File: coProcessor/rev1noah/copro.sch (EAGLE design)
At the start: 97 parts, among them IC1 STM32F405RGT6, J1 USB_MINI-B_SMT, J2 79107-08, J3 693061010911, J4 30320-6002HB, T1 2N2222, T10 2N2222, T2 2N2222, T3 2N2222, T4 2N2222, T5 2N2222, T6 2N2222, T7 2N2222, T8 2N2222, T9 2N2222, U1 LM2597N-5.0, U2 SN65HVD232QD

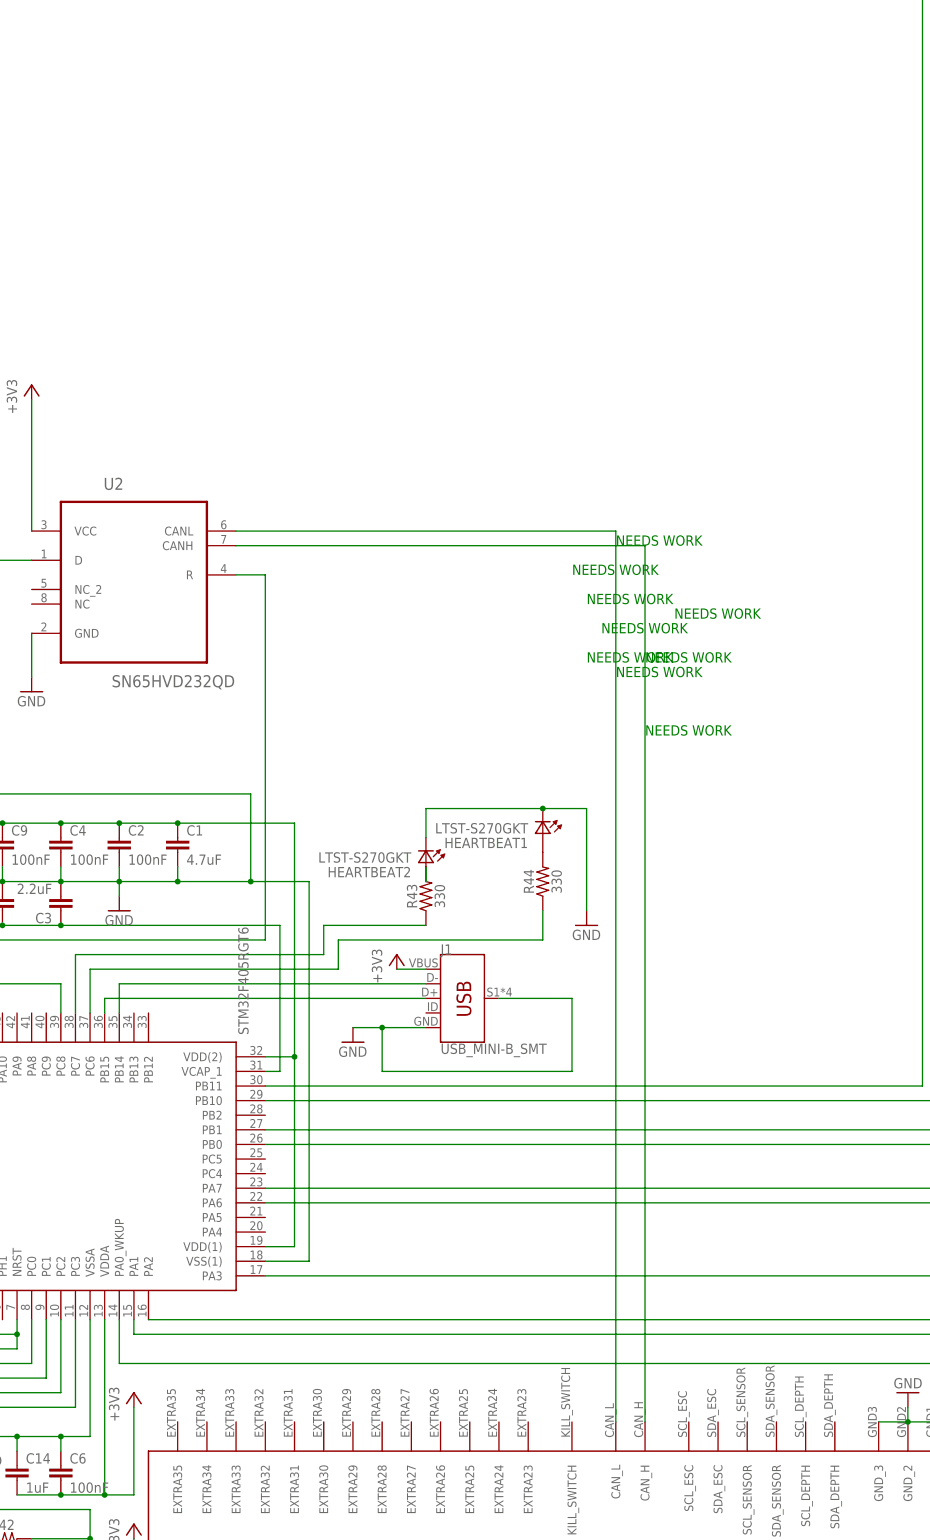
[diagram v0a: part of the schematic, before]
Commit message: Slight progress on last commit, just so everything is up to date
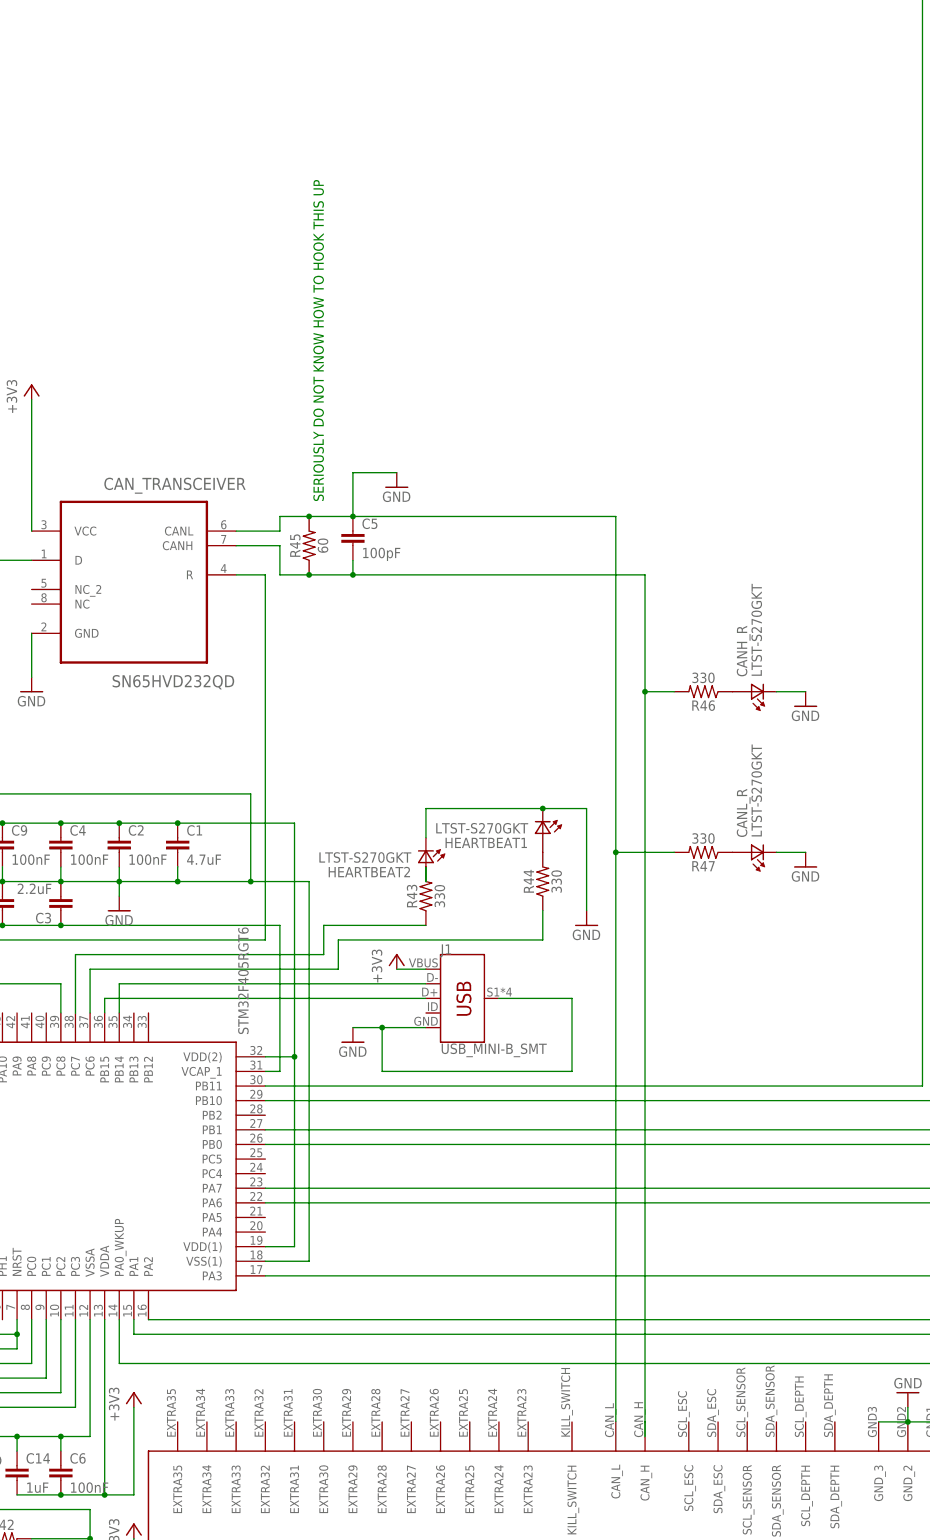
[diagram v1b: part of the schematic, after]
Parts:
- added C5: 100pF, SparkFun-Capacitors:0.1UF-0603-100V-10%
- added CANH_R, CANL_R: LTST-S270GKT, LTST-S270GKT:LTST-S270GKT
- added R45: 60, SparkFun-Resistors:1KOHM-0603-1/10W-1%
- added R46, R47: 330, SparkFun-Resistors:1KOHM-0603-1/10W-1%
- renumbered U2 to CAN_TRANSCEIVER
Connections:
- net N$5 renamed RXD
- removed net N$12: CAN_TRANSCEIVER.CANL, U$1.CAN_L
- new net CANH: C5.2, CAN_TRANSCEIVER.CANH, R45.1, R46.2, U$1.CAN_H
- new net CANL: C5.1, CAN_TRANSCEIVER.CANL, R45.2, R47.2, U$1.CAN_L
- new net N$34: CANH_R.A2, R46.1
- net GND: now also CANH_R.K2, CANL_R.K2
- net N$8: now also CANL_R.A2, R47.1; no longer CAN_TRANSCEIVER.CANH, U$1.CAN_H
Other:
- note added: "SERIOUSLY DO NOT KNOW HOW TO HOOK THIS UP"
- note removed: "NEEDS WORK"
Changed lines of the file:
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@@
 <part name="GND29" library="supply1" library_urn="urn:adsk.eagle:library:371" deviceset="GND" device=""/>
 <part name="+3V3" library="supply1" library_urn="urn:adsk.eagle:library:371" deviceset="+3V3" device=""/>
-<part name="U2" library="SN65HVD232QD" deviceset="SN65HVD232QD" device=""/>
+<part name="CAN_TRANSCEIVER" library="SN65HVD232QD" deviceset="SN65HVD232QD" device=""/>
 <part name="J2" library="con-molex-milli-grid" deviceset="79107-08" device=""/>
 <part name="+3V9" library="supply1" library_urn="urn:adsk.eagle:library:371" deviceset="+3V3" device=""/>
+<part name="R45" library="SparkFun-Resistors" deviceset="1KOHM" device="-0603-1/10W-1%" value="60"/>
+<part name="C5" library="SparkFun-Capacitors" deviceset="0.1UF" device="-0603-100V-10%" value="100pF"/>
+<part name="GND30" library="supply1" library_urn="urn:adsk.eagle:library:371" deviceset="GND" device=""/>
+<part name="R46" library="SparkFun-Resistors" deviceset="1KOHM" device="-0603-1/10W-1%" value="330"/>
+<part name="R47" library="SparkFun-Resistors" deviceset="1KOHM" device="-0603-1/10W-1%" value="330"/>
+<part name="CANL_R" library="LTST-S270GKT" deviceset="LTST-S270GKT" device=""/>
+<part name="CANH_R" library="LTST-S270GKT" deviceset="LTST-S270GKT" device=""/>
+<part name="GND31" library="supply1" library_urn="urn:adsk.eagle:library:371" deviceset="GND" device=""/>
+<part name="GND32" library="supply1" library_urn="urn:adsk.eagle:library:371" deviceset="GND" device=""/>
 </parts>
 <sheets>
@@
 <text x="426.72" y="38.1" size="1.778" layer="91">5 v</text>
 <text x="408.94" y="71.12" size="1.778" layer="91">18 - 22 V</text>
-<text x="279.4" y="226.06" size="1.778" layer="91">NEEDS WORK</text>
-<text x="274.32" y="236.22" size="1.778" layer="91">NEEDS WORK</text>
-<text x="276.86" y="220.98" size="1.778" layer="91">NEEDS WORK</text>
-<text x="287.02" y="208.28" size="1.778" layer="91">NEEDS WORK</text>
-<text x="276.86" y="231.14" size="1.778" layer="91">NEEDS WORK</text>
-<text x="281.94" y="241.3" size="1.778" layer="91">NEEDS WORK</text>
-<text x="292.1" y="228.6" size="1.778" layer="91">NEEDS WORK</text>
-<text x="287.02" y="220.98" size="1.778" layer="91">NEEDS WORK</text>
-<text x="281.94" y="218.44" size="1.778" layer="91">NEEDS WORK</text>
+<text x="231.14" y="248.92" size="1.778" layer="91" rot="R90">SERIOUSLY DO NOT KNOW HOW TO HOOK THIS UP</text>
 </plain>
 <instances>
@@
 <instance part="GND29" gate="1" x="180.34" y="215.9"/>
 <instance part="+3V3" gate="G$1" x="180.34" y="269.24"/>
-<instance part="U2" gate="A" x="198.12" y="238.76"/>
+<instance part="CAN_TRANSCEIVER" gate="A" x="198.12" y="238.76"/>
 <instance part="J2" gate="G$1" x="91.44" y="66.04" rot="R90"/>
 <instance part="+3V9" gate="G$1" x="76.2" y="63.5"/>
+<instance part="R45" gate="G$1" x="228.6" y="241.3" rot="R90"/>
+<instance part="C5" gate="G$1" x="236.22" y="241.3"/>
+<instance part="GND30" gate="1" x="243.84" y="251.46"/>
+<instance part="R46" gate="G$1" x="297.18" y="215.9" rot="R180"/>
+<instance part="R47" gate="G$1" x="297.18" y="187.96" rot="R180"/>
+<instance part="CANL_R" gate="G$1" x="307.34" y="187.96" rot="R90"/>
+<instance part="CANH_R" gate="G$1" x="307.34" y="215.9" rot="R90"/>
+<instance part="GND31" gate="1" x="314.96" y="213.36"/>
+<instance part="GND32" gate="1" x="314.96" y="185.42"/>
 </instances>
 <busses>
@@
 <segment>
 <pinref part="GND29" gate="1" pin="GND"/>
-<pinref part="U2" gate="A" pin="GND"/>
+<pinref part="CAN_TRANSCEIVER" gate="A" pin="GND"/>
 <wire x1="180.34" y1="226.06" x2="180.34" y2="218.44" width="0.1524" layer="91"/>
+</segment>
+<segment>
+<pinref part="CANL_R" gate="G$1" pin="K2"/>
+<pinref part="GND32" gate="1" pin="GND"/>
+<wire x1="309.88" y1="187.96" x2="314.96" y2="187.96" width="0.1524" layer="91"/>
+</segment>
+<segment>
+<pinref part="CANH_R" gate="G$1" pin="K2"/>
+<pinref part="GND31" gate="1" pin="GND"/>
+<wire x1="309.88" y1="215.9" x2="314.96" y2="215.9" width="0.1524" layer="91"/>
 </segment>
 </net>
@@
 <wire x1="180.34" y1="243.84" x2="180.34" y2="266.7" width="0.1524" layer="91"/>
 <pinref part="+3V3" gate="G$1" pin="+3V3"/>
-<pinref part="U2" gate="A" pin="VCC"/>
+<pinref part="CAN_TRANSCEIVER" gate="A" pin="VCC"/>
 </segment>
 <segment>
@@
 <wire x1="160.02" y1="170.18" x2="160.02" y2="238.76" width="0.1524" layer="91"/>
 <wire x1="160.02" y1="238.76" x2="180.34" y2="238.76" width="0.1524" layer="91"/>
-<pinref part="U2" gate="A" pin="D"/>
-</segment>
-</net>
-<net name="N$5" class="0">
+<pinref part="CAN_TRANSCEIVER" gate="A" pin="D"/>
+</segment>
+</net>
+<net name="RXD" class="0">
 <segment>
 <pinref part="IC1" gate="G$1" pin="PA11"/>
@@
 <wire x1="172.72" y1="172.72" x2="220.98" y2="172.72" width="0.1524" layer="91"/>
 <wire x1="220.98" y1="172.72" x2="220.98" y2="236.22" width="0.1524" layer="91"/>
-<pinref part="U2" gate="A" pin="R"/>
+<pinref part="CAN_TRANSCEIVER" gate="A" pin="R"/>
 <wire x1="220.98" y1="236.22" x2="215.9" y2="236.22" width="0.1524" layer="91"/>
-</segment>
-</net>
-<net name="N$8" class="0">
-<segment>
-<pinref part="U$1" gate="G$1" pin="CAN_H"/>
-<pinref part="U2" gate="A" pin="CANH"/>
-<wire x1="287.02" y1="88.9" x2="287.02" y2="241.3" width="0.1524" layer="91"/>
-<wire x1="287.02" y1="241.3" x2="215.9" y2="241.3" width="0.1524" layer="91"/>
-</segment>
-</net>
-<net name="N$12" class="0">
-<segment>
-<pinref part="U$1" gate="G$1" pin="CAN_L"/>
-<pinref part="U2" gate="A" pin="CANL"/>
-<wire x1="281.94" y1="88.9" x2="281.94" y2="243.84" width="0.1524" layer="91"/>
-<wire x1="281.94" y1="243.84" x2="215.9" y2="243.84" width="0.1524" layer="91"/>
 </segment>
 </net>
@@
 </segment>
 </net>
+<net name="CANH" class="0">
+<segment>
+<pinref part="R45" gate="G$1" pin="1"/>
+<pinref part="C5" gate="G$1" pin="2"/>
+<wire x1="228.6" y1="236.22" x2="236.22" y2="236.22" width="0.1524" layer="91"/>
+<wire x1="236.22" y1="236.22" x2="236.22" y2="238.76" width="0.1524" layer="91"/>
+<wire x1="228.6" y1="236.22" x2="223.52" y2="236.22" width="0.1524" layer="91"/>
+<junction x="228.6" y="236.22"/>
+<wire x1="223.52" y1="236.22" x2="223.52" y2="241.3" width="0.1524" layer="91"/>
+<pinref part="CAN_TRANSCEIVER" gate="A" pin="CANH"/>
+<wire x1="223.52" y1="241.3" x2="215.9" y2="241.3" width="0.1524" layer="91"/>
+<wire x1="236.22" y1="236.22" x2="287.02" y2="236.22" width="0.1524" layer="91"/>
+<junction x="236.22" y="236.22"/>
+<pinref part="U$1" gate="G$1" pin="CAN_H"/>
+<wire x1="287.02" y1="236.22" x2="287.02" y2="215.9" width="0.1524" layer="91"/>
+<wire x1="287.02" y1="215.9" x2="287.02" y2="88.9" width="0.1524" layer="91"/>
+<wire x1="287.02" y1="86.36" x2="287.02" y2="88.9" width="0.1524" layer="91"/>
+<pinref part="R46" gate="G$1" pin="2"/>
+<wire x1="292.1" y1="215.9" x2="287.02" y2="215.9" width="0.1524" layer="91"/>
+<junction x="287.02" y="215.9"/>
+</segment>
+</net>
+<net name="N$8" class="0">
+<segment>
+<pinref part="R47" gate="G$1" pin="1"/>
+<pinref part="CANL_R" gate="G$1" pin="A2"/>
+</segment>
+</net>
+<net name="N$34" class="0">
+<segment>
+<pinref part="R46" gate="G$1" pin="1"/>
+<pinref part="CANH_R" gate="G$1" pin="A2"/>
+</segment>
+</net>
+<net name="CANL" class="0">
+<segment>
+<pinref part="R45" gate="G$1" pin="2"/>
+<pinref part="C5" gate="G$1" pin="1"/>
+<wire x1="228.6" y1="246.38" x2="236.22" y2="246.38" width="0.1524" layer="91"/>
+<pinref part="CAN_TRANSCEIVER" gate="A" pin="CANL"/>
+<wire x1="215.9" y1="243.84" x2="223.52" y2="243.84" width="0.1524" layer="91"/>
+<wire x1="223.52" y1="243.84" x2="223.52" y2="246.38" width="0.1524" layer="91"/>
+<wire x1="223.52" y1="246.38" x2="228.6" y2="246.38" width="0.1524" layer="91"/>
+<junction x="228.6" y="246.38"/>
+<pinref part="U$1" gate="G$1" pin="CAN_L"/>
+<wire x1="281.94" y1="88.9" x2="281.94" y2="187.96" width="0.1524" layer="91"/>
+<wire x1="281.94" y1="187.96" x2="281.94" y2="246.38" width="0.1524" layer="91"/>
+<wire x1="281.94" y1="246.38" x2="236.22" y2="246.38" width="0.1524" layer="91"/>
+<junction x="236.22" y="246.38"/>
+<pinref part="GND30" gate="1" pin="GND"/>
+<wire x1="236.22" y1="246.38" x2="236.22" y2="254" width="0.1524" layer="91"/>
+<wire x1="236.22" y1="254" x2="243.84" y2="254" width="0.1524" layer="91"/>
+<pinref part="R47" gate="G$1" pin="2"/>
+<wire x1="292.1" y1="187.96" x2="281.94" y2="187.96" width="0.1524" layer="91"/>
+<junction x="281.94" y="187.96"/>
+</segment>
+</net>
